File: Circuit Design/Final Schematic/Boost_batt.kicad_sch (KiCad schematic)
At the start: 0 parts

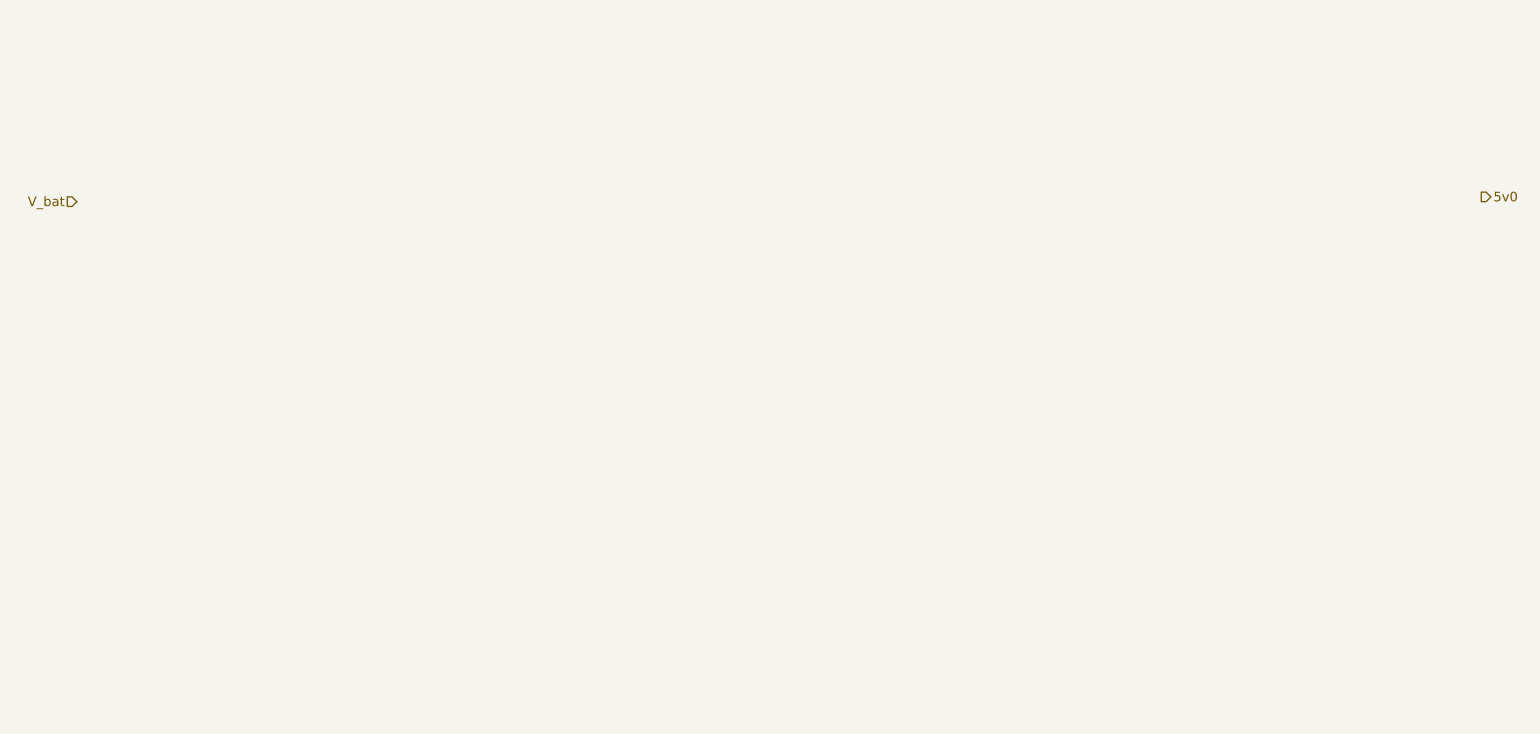
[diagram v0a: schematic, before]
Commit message: Boost
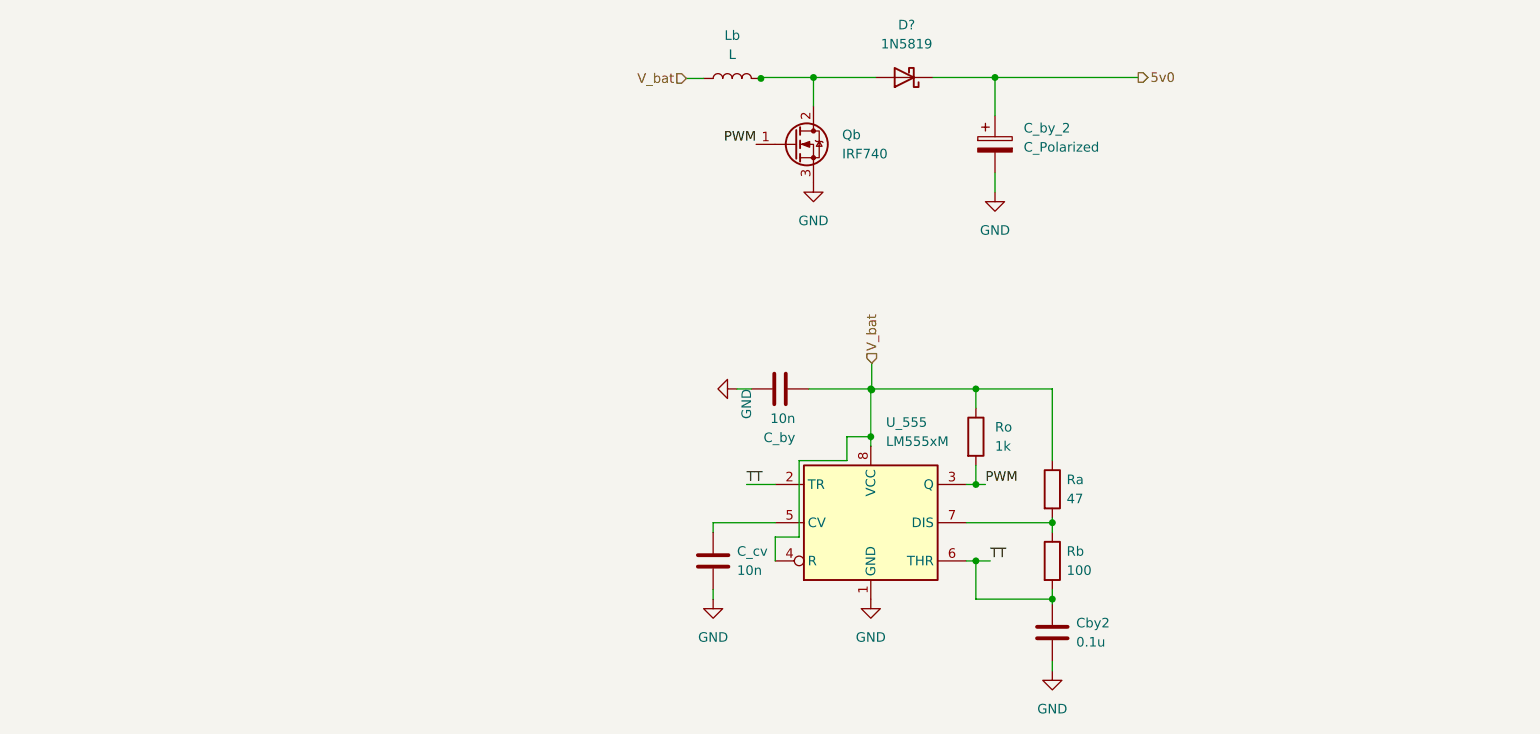
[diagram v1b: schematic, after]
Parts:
- added C_by, C_cv: 10n, Capacitor_SMD:C_0805_2012Metric_Pad1.18x1.45mm_HandSolder, symbol Device:C
- added C_by_2: C_Polarized, symbol Device:C_Polarized
- added Cby2: 0.1u, Capacitor_SMD:C_0805_2012Metric_Pad1.18x1.45mm_HandSolder, symbol Device:C
- added D?: 1N5819, Diode_THT:D_DO-41_SOD81_P10.16mm_Horizontal, symbol Diode:1N5819
- added Lb: L, symbol Device:L
- added Qb: IRF740, Package_TO_SOT_THT:TO-220-3_Vertical, symbol Transistor_FET:IRF740
- added Ra: 47, symbol Device:R
- added Rb: 100, Resistor_SMD:R_0805_2012Metric_Pad1.20x1.40mm_HandSolder, symbol Device:R
- added Ro: 1k, symbol Device:R
- added U_555: LM555xM, Package_SO:SOIC-8_3.9x4.9mm_P1.27mm, symbol Timer:LM555xM
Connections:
- net 5v0: now also C_by_2.1, D?.1 (K)
- net V_bat: now also Lb.1
- new net: C_by.2, Ra.1, Ro.1, U_555.4 (R), U_555.8 (VCC)
- new net: D?.2 (A), Qb.2 (D)
- new net: Ra.2, Rb.1, U_555.7 (DIS)
- new net: C_cv.1, U_555.5 (CV)
- new net GND: C_by.1, C_by_2.2, C_cv.2, Cby2.2, Qb.3 (S), U_555.1 (GND)
- new net PWM: Qb.1 (G), Ro.2, U_555.3 (Q)
- new net TT: Cby2.1, Rb.2, U_555.2 (TR), U_555.6 (THR)
